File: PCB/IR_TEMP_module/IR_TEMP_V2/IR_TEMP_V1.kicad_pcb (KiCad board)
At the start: 2 copper layers, 10 x 20 mm, 26 parts, among them IC1 LMP91051MTX_NOPB, J1 1_PIN, J10 1_PIN, J11 1_PIN, J12 1_PIN, J2 1_PIN, J3 1_PIN, J4 1_PIN, J5 1_PIN, J6 1_PIN, J7 1_PIN, J8 1_PIN, J9 1_PIN, U1 ZTP-135SR

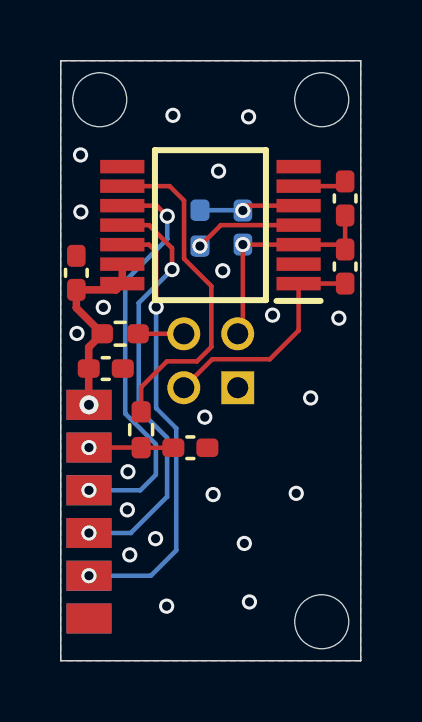
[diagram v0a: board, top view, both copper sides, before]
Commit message: udated by FZ
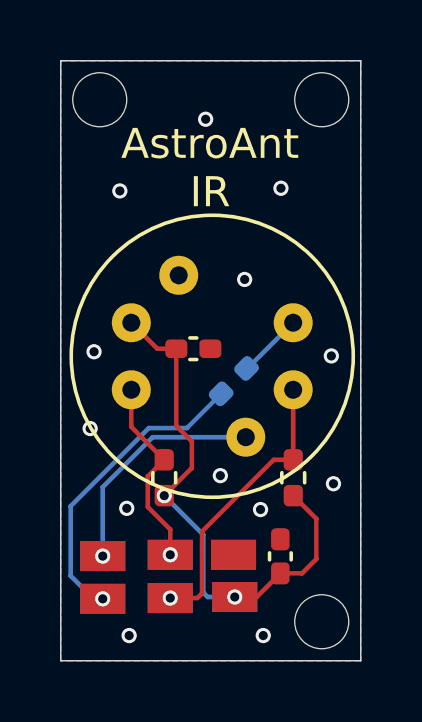
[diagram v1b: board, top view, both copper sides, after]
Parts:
- removed C3, C4: 0.01uF, Capacitor_SMD:C_0402_1005Metric_Pad0.74x0.62mm_HandSolder
- removed C5: 1uF, Capacitor_SMD:C_0402_1005Metric_Pad0.74x0.62mm_HandSolder
- removed C6: 6800pF, Capacitor_SMD:C_0402_1005Metric_Pad0.74x0.62mm_HandSolder
- removed IC1: LMP91051MTX_NOPB, SamacSys_Parts:SOP65P640X120-14N
- R2, R3: value 160k -> 100k
- U1: value ZTP-135SR -> TPIS_1T_1084; footprint Mylib:TO-46-4 -> Mylib:TPIS_1T_1084; moved to F.Cu
- moved C1 8.55 mm to (116.3, 70.5), turned to 270 degrees
- moved J1 8.04 mm to (114.8, 69.9)
- moved J7 8.04 mm to (114.8, 73.9)
- moved J10 5.70 mm to (112.7, 73.9)
- moved J4 5.70 mm to (112.7, 69.9)
- moved R2 5.32 mm to (116.8, 67.9), turned to 270 degrees
- moved J2 5.27 mm to (114.8, 68.5)
- moved J8 5.27 mm to (114.8, 72.5)
- moved R3 5.22 mm to (114.8, 64.7), turned to 225 degrees
- moved R1 5.02 mm to (112.5, 67.9), turned to 270 degrees
- moved C2 4.65 mm to (113.4, 63.6), turned to 180 degrees
- moved J3 3.46 mm to (112.7, 68.5)
- moved J9 3.46 mm to (112.7, 72.6)
- moved J11 0.90 mm to (110.4, 72.5)
- moved J12 0.90 mm to (110.4, 73.9)
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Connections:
- J10 pad 1: /Temp_A -> /SCL
- J11 pad 1: /SCLK -> /A1
- J12 pad 1: /MOSI -> /INT
- J3 pad 1: /SPICS -> /SDA
- J4 pad 1: /Temp_A -> /SCL
- J5 pad 1: /SCLK -> /A1
- J6 pad 1: /MOSI -> /INT
- J9 pad 1: /SPICS -> /SDA
- R1 pad 1: +3V3 -> /SDA
- R1 pad 2: /Thermistor -> +3V3
- R2 pad 1: /Temp_A -> /SCL
- R2 pad 2: Net-(IC1-Pad9) -> +3V3
- R3 pad 1: /A1 -> /INT_TPIS
- R3 pad 2: /A0 -> /INT
- U1 pad 2: Net-(C3-Pad2) -> +3V3
- U1 pad 3: /Thermistor -> /SDA
- U1 pad 4: /CMOUT -> /INT_TPIS
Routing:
- net /MOSI: track 14.7 -> 0.00 mm, vias 2 -> 0
- net /SCLK: track 14.2 -> 0.00 mm, vias 2 -> 0
- net /SPICS: track 13.7 -> 0.00 mm, vias 2 -> 0
- net +3V3: track 6.65 -> 17.9 mm, vias 1 -> 2
- net Net-(IC1-Pad9): track 11.2 -> 0.00 mm
- net /INT: track 0.00 -> 10.3 mm, vias 0 -> 1
- net /SCL: track 0.00 -> 9.55 mm, vias 0 -> 1
- net Net-(C3-Pad2): track 7.73 -> 0.00 mm
- net /CMOUT: track 7.66 -> 0.00 mm, vias 1 -> 0
- net /SDA: track 0.00 -> 6.49 mm, vias 0 -> 1
- net /A1: track 3.36 -> 7.76 mm
- net /A0: track 3.58 -> 0.00 mm, vias 1 -> 0
- net /Temp_A: track 2.81 -> 0.00 mm, vias 1 -> 0
- net /INT_TPIS: track 0.00 -> 2.19 mm
- net GND: track 1.62 -> 0.00 mm, vias 21 -> 13
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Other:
- board text added: "AstroAnt IR"
